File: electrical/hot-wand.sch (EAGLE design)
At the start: 203 parts, among them IC1 12V R-78K12-2.0, IC2 3V3 R-78K3.3, Q1 STP19NF20, Q2 IRF510, Q3 BC846B, Q4 SIS862ADN-T1-GE3, Q5 SIS862ADN-T1-GE3, Q6 DMTH64M2LPDWQ-13, Q7 SIS862ADN-T1-GE3, Q8 2N7002K, Q9 G3404, SW1 SW-TACT-SIDE, U1 TPS54560DDA, U2 1EDN8511BXUSA1, U3 STM32F030F4P6, U4 SSD1306-4PIN-0.91N-VERT, U5 INA138, U6 LM74810QDRRRQ1, U7 AP53781, Y1 27.12 MHz 10pF

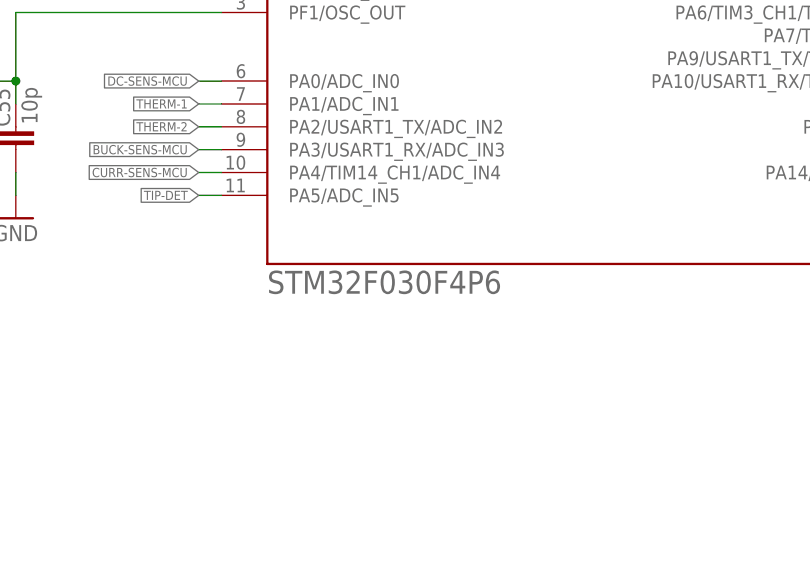
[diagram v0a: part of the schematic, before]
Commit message: part num update
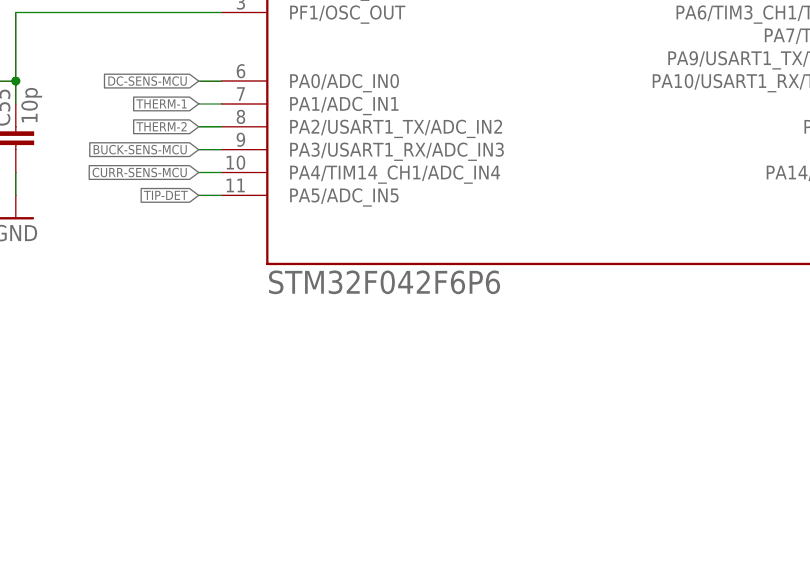
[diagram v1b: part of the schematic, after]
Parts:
- U3: value STM32F030F4P6 -> STM32F042F6P6
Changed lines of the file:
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@@
 <attribute name="JLC-DNP" value="1"/>
 </part>
-<part name="U3" library="hot-wand" deviceset="STM32F030F4P6" device="">
+<part name="U3" library="hot-wand" deviceset="STM32F030F4P6" device="" value="STM32F042F6P6">
 <attribute name="JLCPARTNUM" value="C2969989"/>
 <attribute name="JLC_ROTATION" value="180"/>
